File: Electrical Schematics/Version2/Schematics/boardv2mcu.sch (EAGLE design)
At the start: 12 parts, among them U1 TMS570LS0432_PZ_100

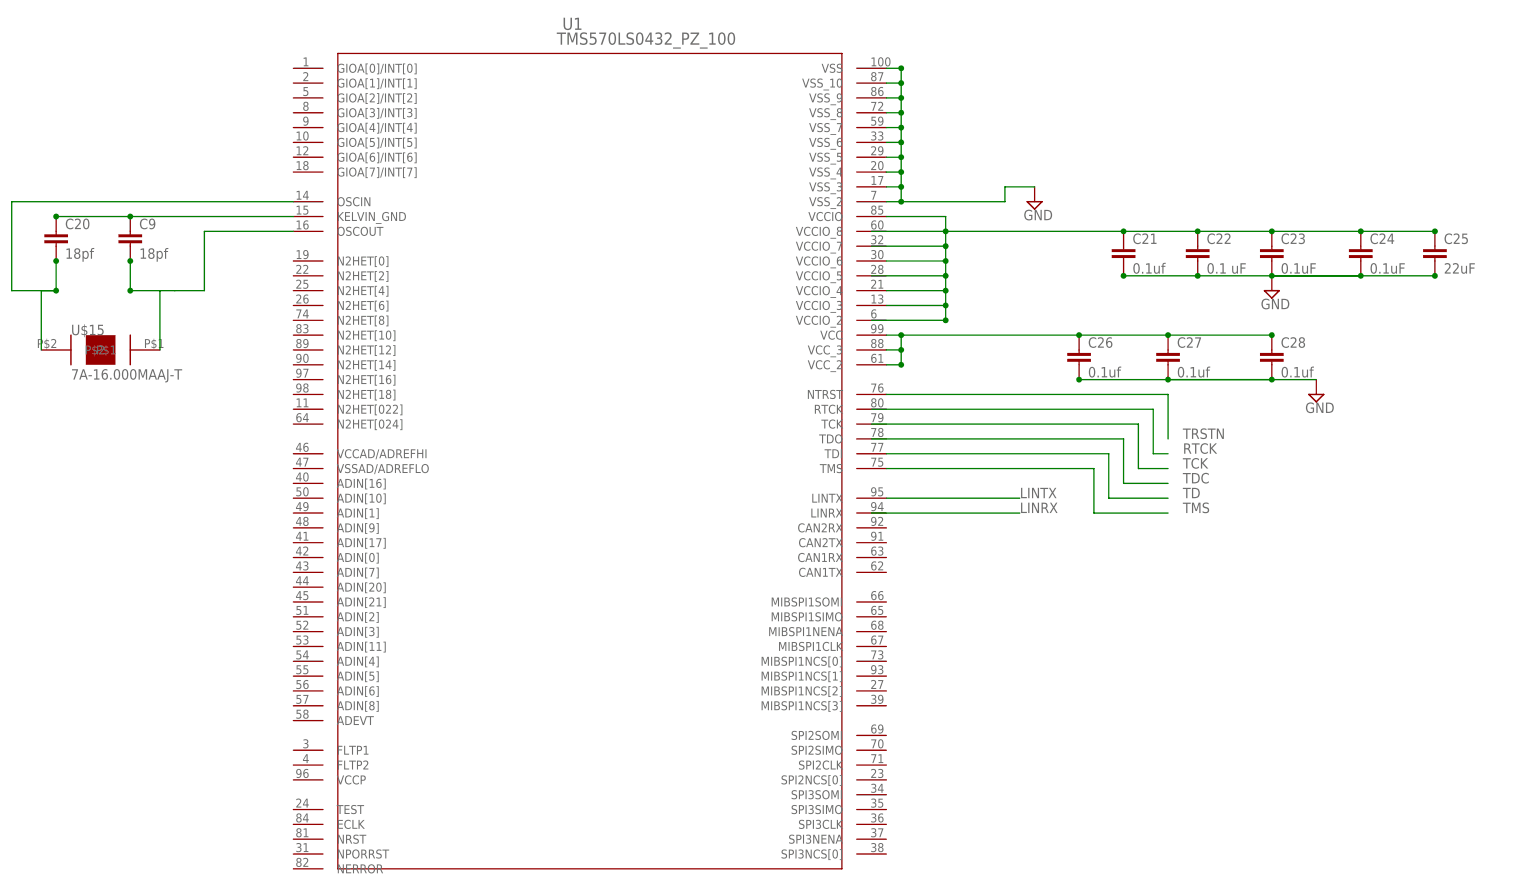
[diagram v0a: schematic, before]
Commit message: MCU JTAG
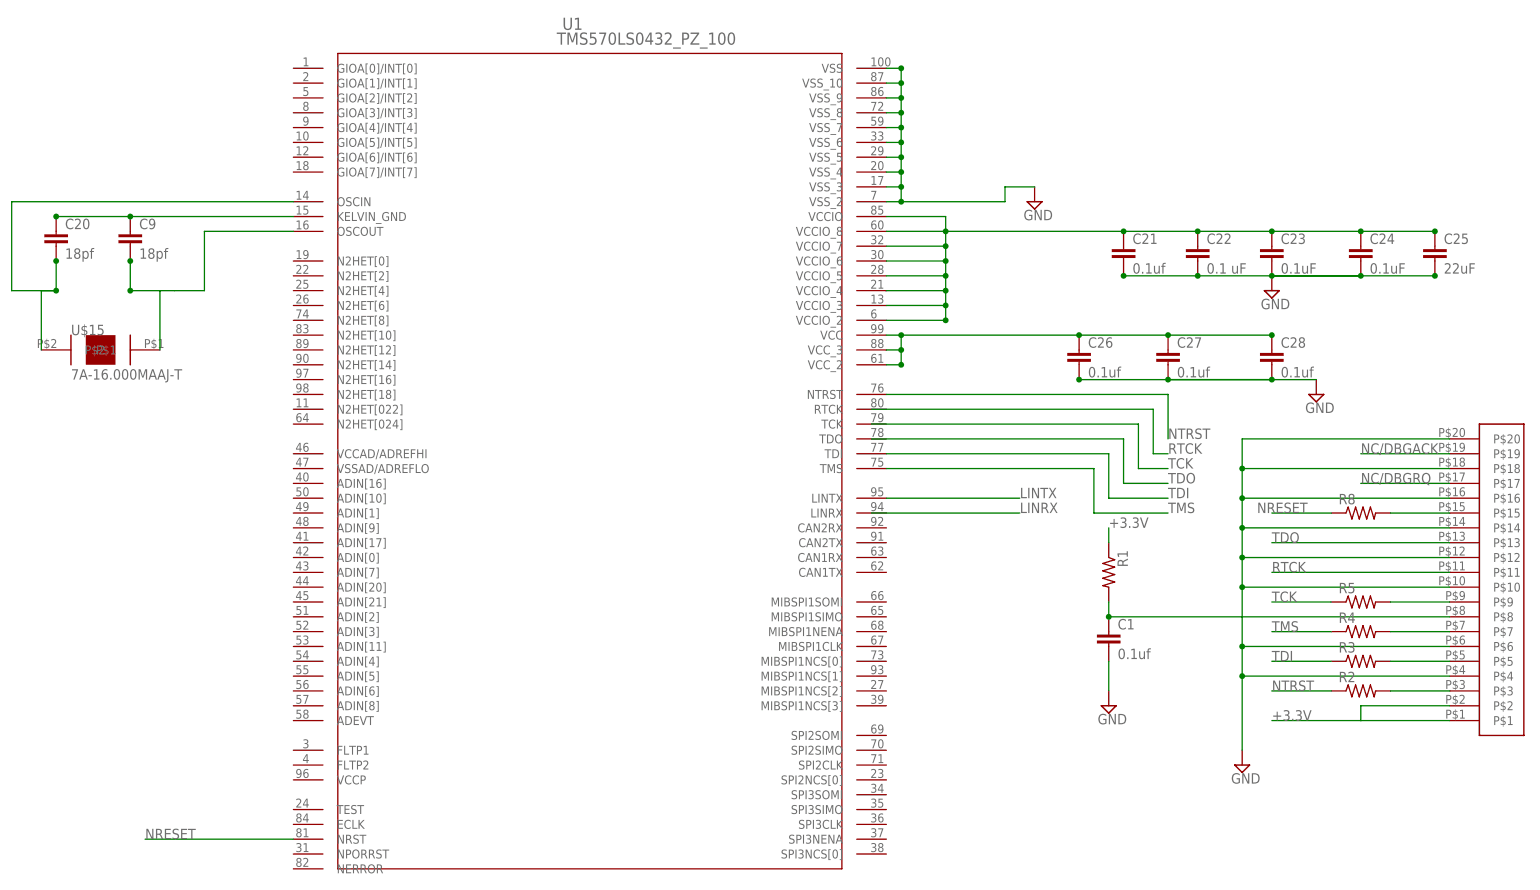
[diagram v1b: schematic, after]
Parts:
- added C1: 0.1uf, rcl:C-EUC0603
- added R1, R2, R3, R4, R5, R8: (no value), SparkFun-Passives:RESISTOR0603-RES
- added U$1: JTAG20PIN, connectors:JTAG20PIN
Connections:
- removed net TD: U1.TDI
- removed net TRSTN: U1.NTRST
- new net +3.3V: R1.1, U$1.P$1, U$1.P$2
- new net N$1: C1.1, R1.2, U$1.P$8
- new net NC/DBGACK: U$1.P$19
- new net NC/DBGRQ: U$1.P$17
- new net NRESET: R8.1, R8.2, U$1.P$15, U1.NRST
- new net NTRST: R2.1, R2.2, U$1.P$3, U1.NTRST
- new net RTCK: U$1.P$11
- new net TCK: R5.1, R5.2, U$1.P$9
- new net TDI: R3.1, R3.2, U$1.P$5, U1.TDI
- new net TDO: U$1.P$13
- net GND: now also C1.2, U$1.P$10, U$1.P$12, U$1.P$14, U$1.P$16, U$1.P$18, U$1.P$20, U$1.P$4, U$1.P$6
- net TMS: now also R4.1, R4.2, U$1.P$7
